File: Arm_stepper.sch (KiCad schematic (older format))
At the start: 125 parts, among them IC1 L6208D, IC2 L6208D, J1 12V_CONN, J10 ENCODER1, J11 ENCODER2, J2 M1_CONN, J3 M1_CONN, J4 Conn_01x06_Male, J5 I2C_CONN, J6 SWDCONNUSART, J8 Conn_01x04_Female, J9 USB_B_Mini, M2 Fan, Q2 2N2219, SW1 SW_Push_Dual, SW2 endstop4, SW3 endstop1, SW4 endstop3, SW5 endstop2, U1 ISO1050-00_isolation, U2 USBLC6-2SC6, U3 STM32F446RETx, U4 LM1117-3.3, U5 LM1117-5, Y1 8Mhz

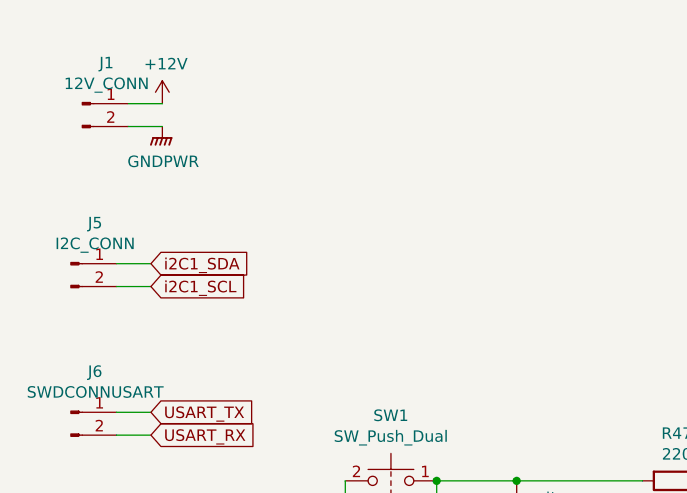
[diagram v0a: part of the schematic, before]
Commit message: finished
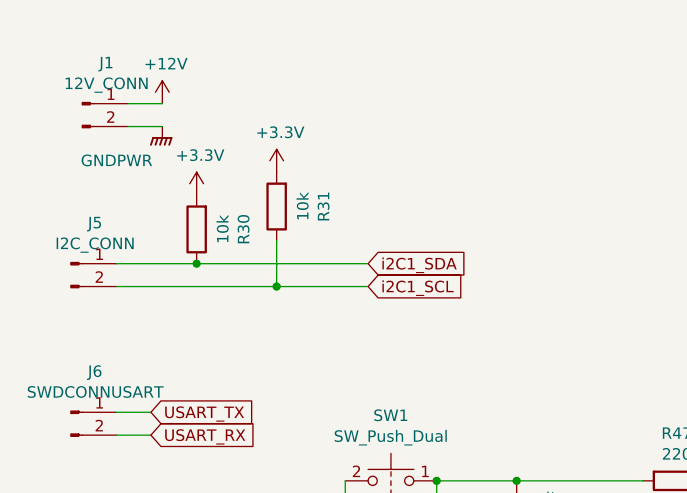
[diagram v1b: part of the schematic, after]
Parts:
- added R30, R31: 10k, Resistor_SMD:R_0805_2012Metric, symbol Device:R
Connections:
- net +3V3: now also R30.2, R31.2
- net i2C1_SCL: now also R31.1
- net i2C1_SDA: now also R30.1
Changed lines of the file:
@@
 Wire Wire Line
 	3600 9950 3800 9950
-Wire Wire Line
-	850  1650 1000 1650
-Wire Wire Line
-	850  1550 1000 1550
 $Comp
 L Connector:Conn_01x02_Male J5
@@
 	1    0    0    -1
 $EndComp
-Text GLabel 1000 1550 2    50   Input ~ 0
+Text GLabel 1950 1550 2    50   Input ~ 0
 i2C1_SDA
-Text GLabel 1000 1650 2    50   Input ~ 0
+Text GLabel 1950 1650 2    50   Input ~ 0
 i2C1_SCL
 $Comp
@@
 P 1050 950
 F 0 "#PWR0107" H 1050 750 50  0001 C CNN
-F 1 "GNDPWR" H 1054 796 50  0000 C CNN
+F 1 "GNDPWR" H 850 800 50  0000 C CNN
 F 2 "" H 1050 900 50  0001 C CNN
 F 3 "" H 1050 900 50  0001 C CNN
@@
 Wire Wire Line
 	3400 3950 4000 3950
+$Comp
+L Device:R R30
+U 1 1 5C853947
+P 1200 1400
+F 0 "R30" V 993 1400 50  0000 C CNN
+F 1 "10k" V 1084 1400 50  0000 C CNN
+F 2 "Resistor_SMD:R_0805_2012Metric" V 1130 1400 50  0001 C CNN
+F 3 "~" H 1200 1400 50  0001 C CNN
+	1    1200 1400
+	-1   0    0    1
+$EndComp
+$Comp
+L Device:R R31
+U 1 1 5C85521B
+P 1550 1300
+F 0 "R31" V 1343 1300 50  0000 C CNN
+F 1 "10k" V 1434 1300 50  0000 C CNN
+F 2 "Resistor_SMD:R_0805_2012Metric" V 1480 1300 50  0001 C CNN
+F 3 "~" H 1550 1300 50  0001 C CNN
+	1    1550 1300
+	-1   0    0    1
+$EndComp
+Wire Wire Line
+	850  1550 1200 1550
+Wire Wire Line
+	1200 1550 1950 1550
+Connection ~ 1200 1550
+Wire Wire Line
+	850  1650 1550 1650
+Wire Wire Line
+	1550 1450 1550 1650
+Connection ~ 1550 1650
+Wire Wire Line
+	1550 1650 1950 1650
+$Comp
+L power:+3.3V #PWR0112
+U 1 1 5C8EB3CB
+P 1200 1250
+F 0 "#PWR0112" H 1200 1100 50  0001 C CNN
+F 1 "+3.3V" H 1215 1423 50  0000 C CNN
+F 2 "" H 1200 1250 50  0001 C CNN
+F 3 "" H 1200 1250 50  0001 C CNN
+	1    1200 1250
+	1    0    0    -1
+$EndComp
+$Comp
+L power:+3.3V #PWR0114
+U 1 1 5C8EBE5F
+P 1550 1150
+F 0 "#PWR0114" H 1550 1000 50  0001 C CNN
+F 1 "+3.3V" H 1565 1323 50  0000 C CNN
+F 2 "" H 1550 1150 50  0001 C CNN
+F 3 "" H 1550 1150 50  0001 C CNN
+	1    1550 1150
+	1    0    0    -1
+$EndComp
 $EndSCHEMATC
